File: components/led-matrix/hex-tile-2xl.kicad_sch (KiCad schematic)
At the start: 58 parts, among them J1 Conn_01x04_Socket, J2 USB_B_Micro, Q1 NPN, Q2 NPN, U1 ESP32-C3-MINI-1, U10 CP2102C-Axx-xQFN24, U3 AP2112K-3.3, U5 MCP23017x-x-SO, U8 171050601

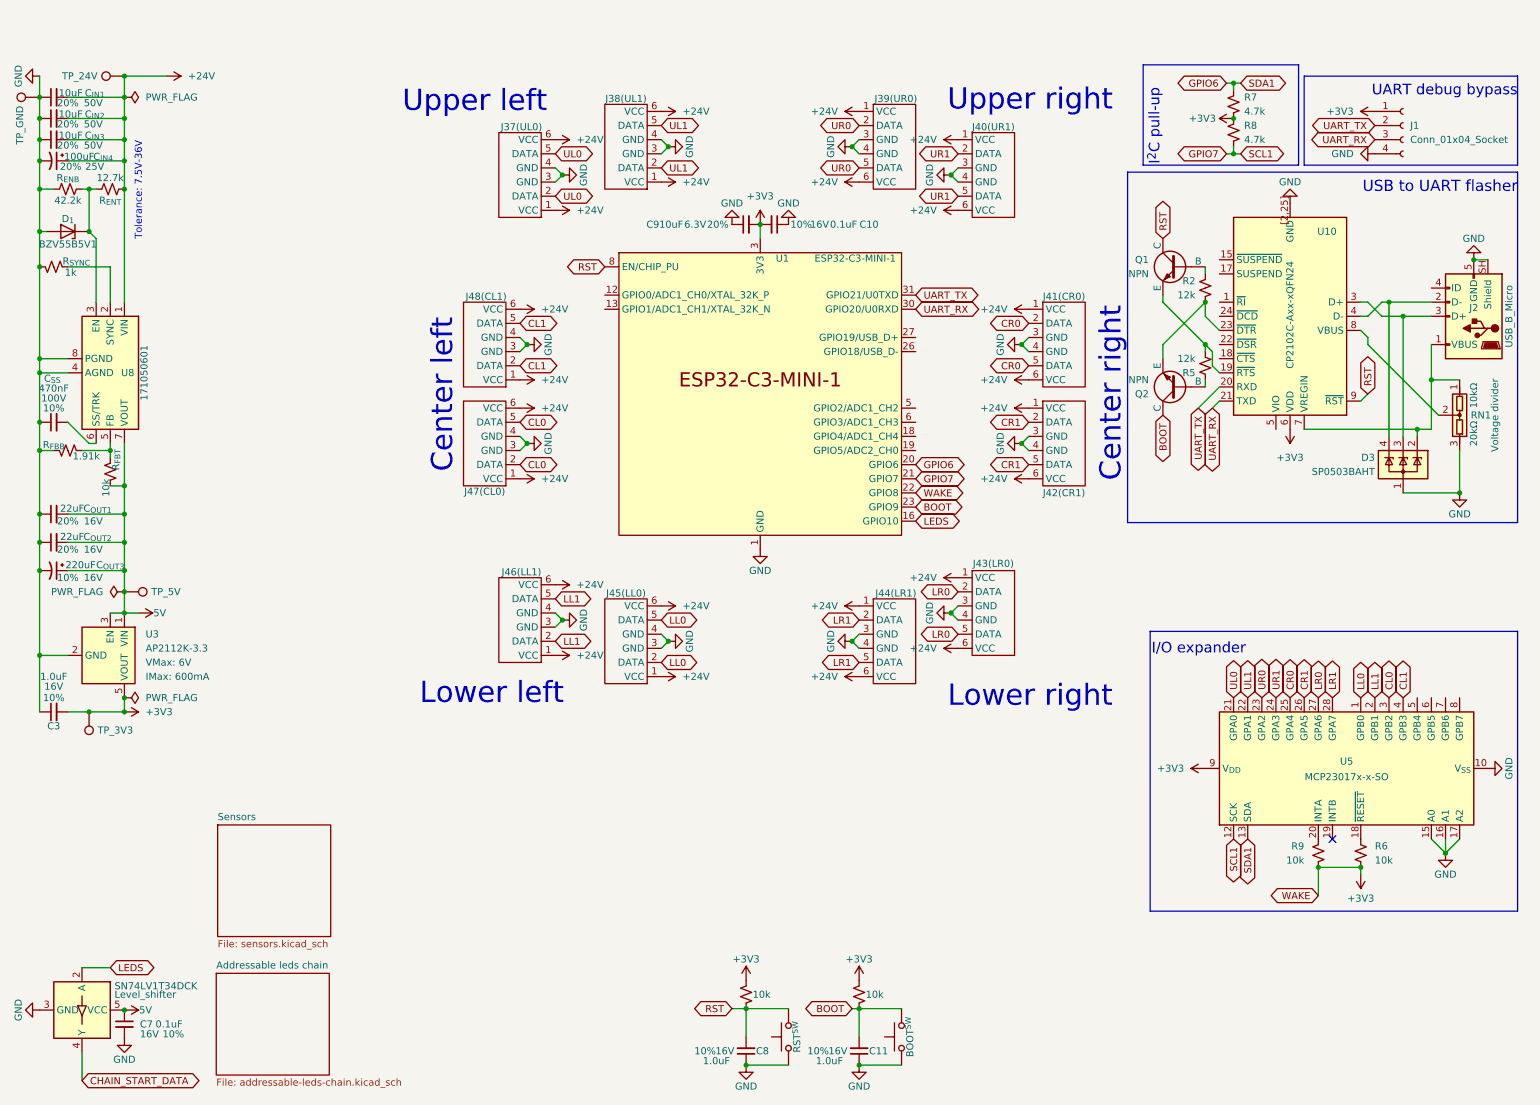
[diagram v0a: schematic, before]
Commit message: svg
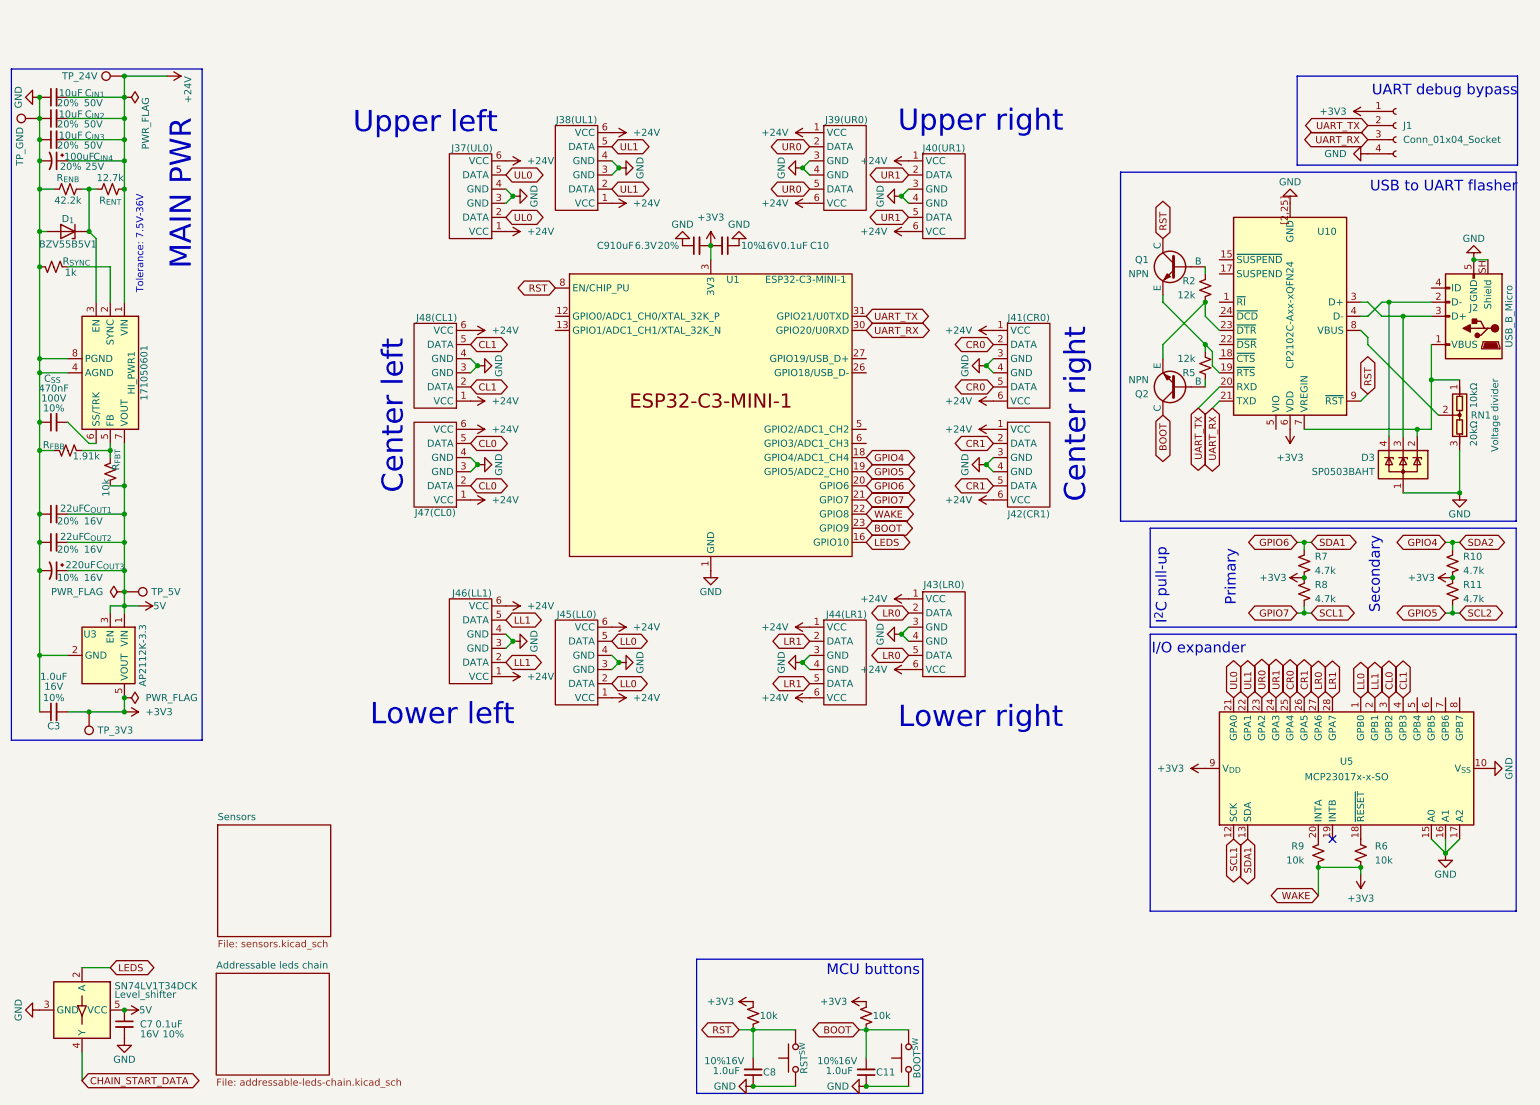
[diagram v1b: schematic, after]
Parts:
- added R10, R11: 4.7k, PCM_SparkFun-Resistor:R_0402_1005Metric, symbol PCM_SparkFun-Resistor:4.7k_0402
- renumbered U8 to HI_PWR1
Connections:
- net +3V3: now also R10.2, R11.2
- net GPIO4: now reaches U1.18 (GPIO4/ADC1_CH4)
- net GPIO4: now also R10.1
- net GPIO5: now reaches U1.19 (GPIO5/ADC2_CH0)
- net GPIO5: now also R11.1
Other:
- note added: "MAIN PWR"
- note added: "MCU buttons"
- note added: "Primary"
- note added: "Secondary"
- moved on the sheet: BOOT^{SW}, C10, C11, C8, C9, J1, J37(UL0), J38(UL1), J39(UR0), J40(UR1), J41(CR0), J42(CR1)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
